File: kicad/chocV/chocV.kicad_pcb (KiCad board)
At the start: 2 copper layers, 212.5 x 78.7 mm, 83 parts, among them SW1 SW_Push, SW10 SW_Push, SW11 SW_Push, SW12 SW_Push, SW13 SW_Push, SW14 SW_Push, SW15 SW_Push, SW16 SW_Push, SW17 SW_Push, SW18 SW_Push, SW19 SW_Push, SW2 SW_Push, SW20 SW_Push, SW21 SW_Push, SW22 SW_Push, SW23 SW_Push, SW24 SW_Push, SW25 SW_Push, SW26 SW_Push, SW27 SW_Push, SW28 SW_Push, SW29 SW_Push, SW3 SW_Push, SW30 SW_Push, SW31 SW_Push, SW32 SW_Push, SW33 SW_Push, SW34 SW_Push, SW35 SW_Push, SW36 SW_Push, SW37 Reset Switch, SW4 SW_Push, SW5 SW_Push, SW6 SW_Push, SW7 SW_Push, SW8 SW_Push, SW9 SW_Push, U1 Pro-Micro

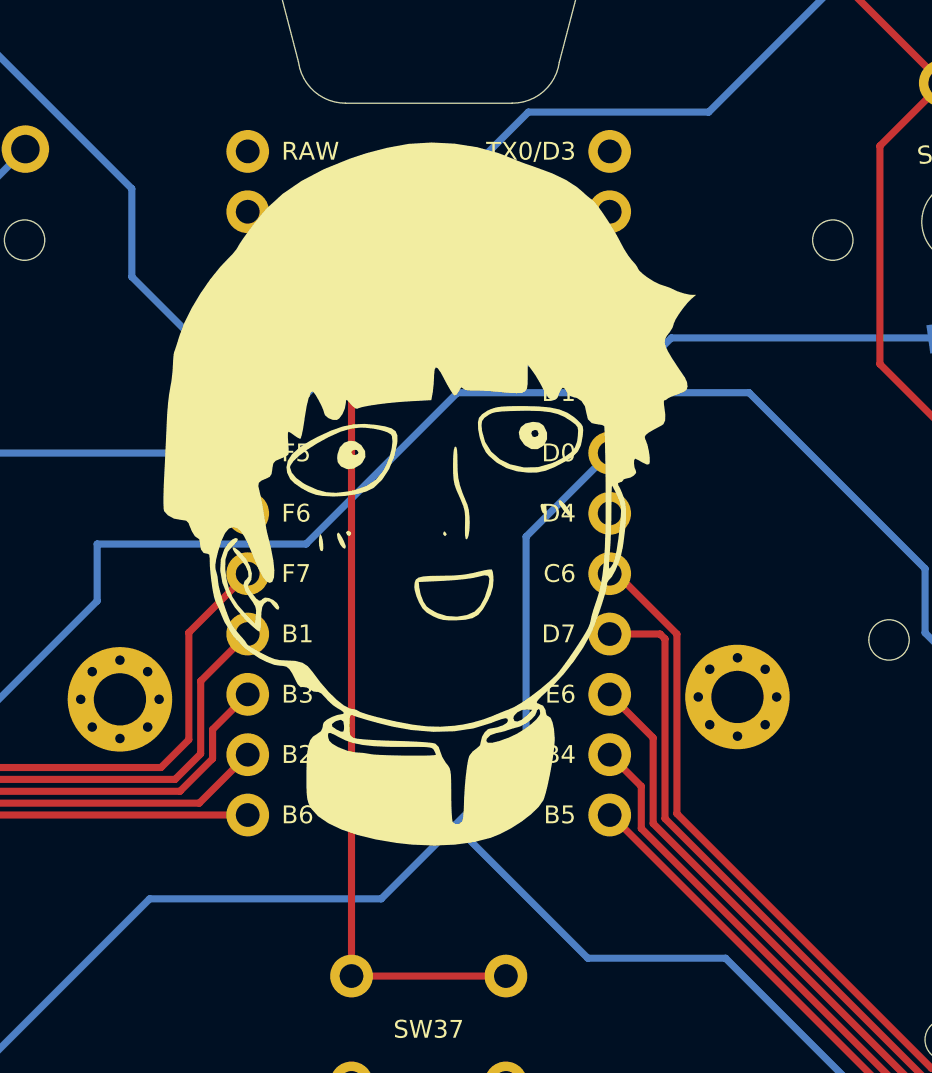
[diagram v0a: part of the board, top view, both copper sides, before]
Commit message: new gerbers added
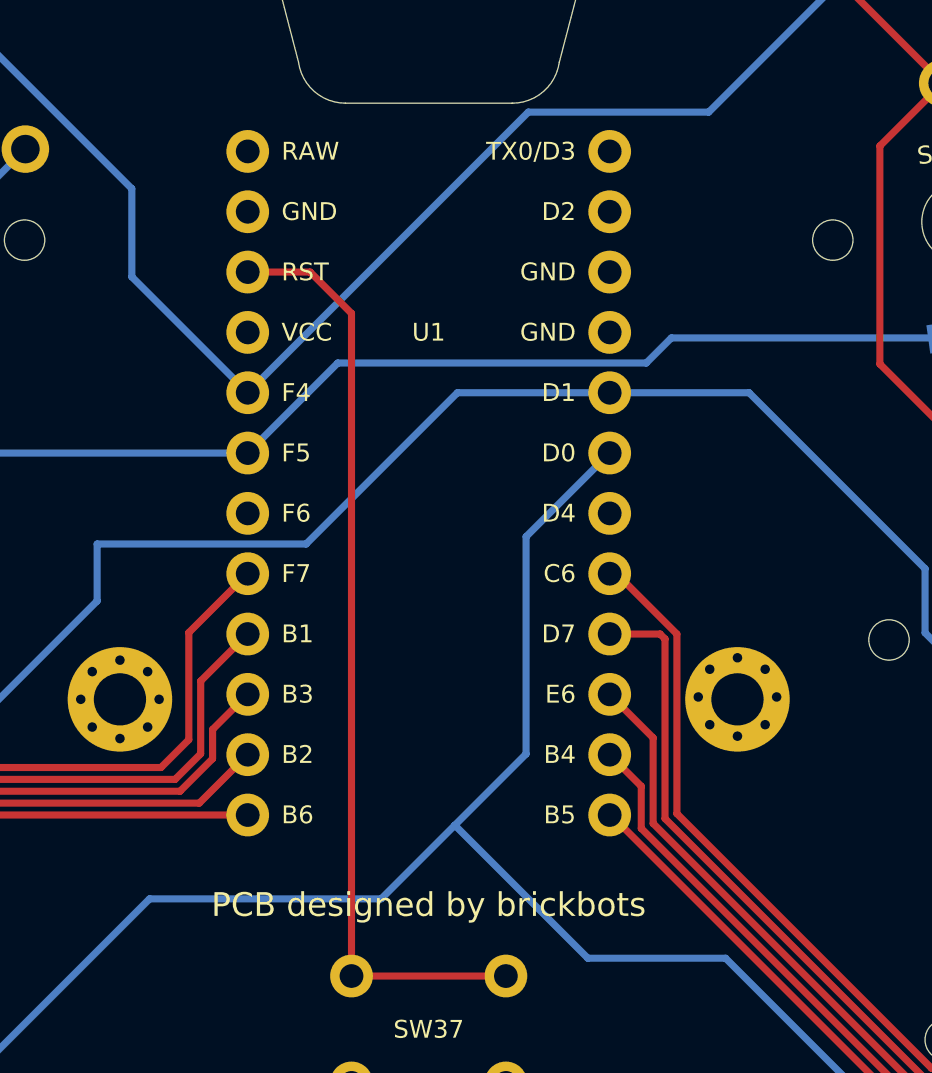
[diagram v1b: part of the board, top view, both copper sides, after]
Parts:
- removed G***: LOGO, KeebGraphics:HappyShigeoSilk
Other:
- board text added: "MOB V 30%"
- board text added: "PCB designed by brickbots"
